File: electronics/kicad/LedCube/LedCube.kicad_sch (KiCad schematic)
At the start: 20 parts, among them J1 Conn_01x03, J2 Conn_01x03, J3 Conn_01x03, J4 Conn_01x04, J5 COM, J6 Conn_01x02, J7 JTAG, U1 ESP32-S3-DevKitC, U3 ESP32-DevKitM

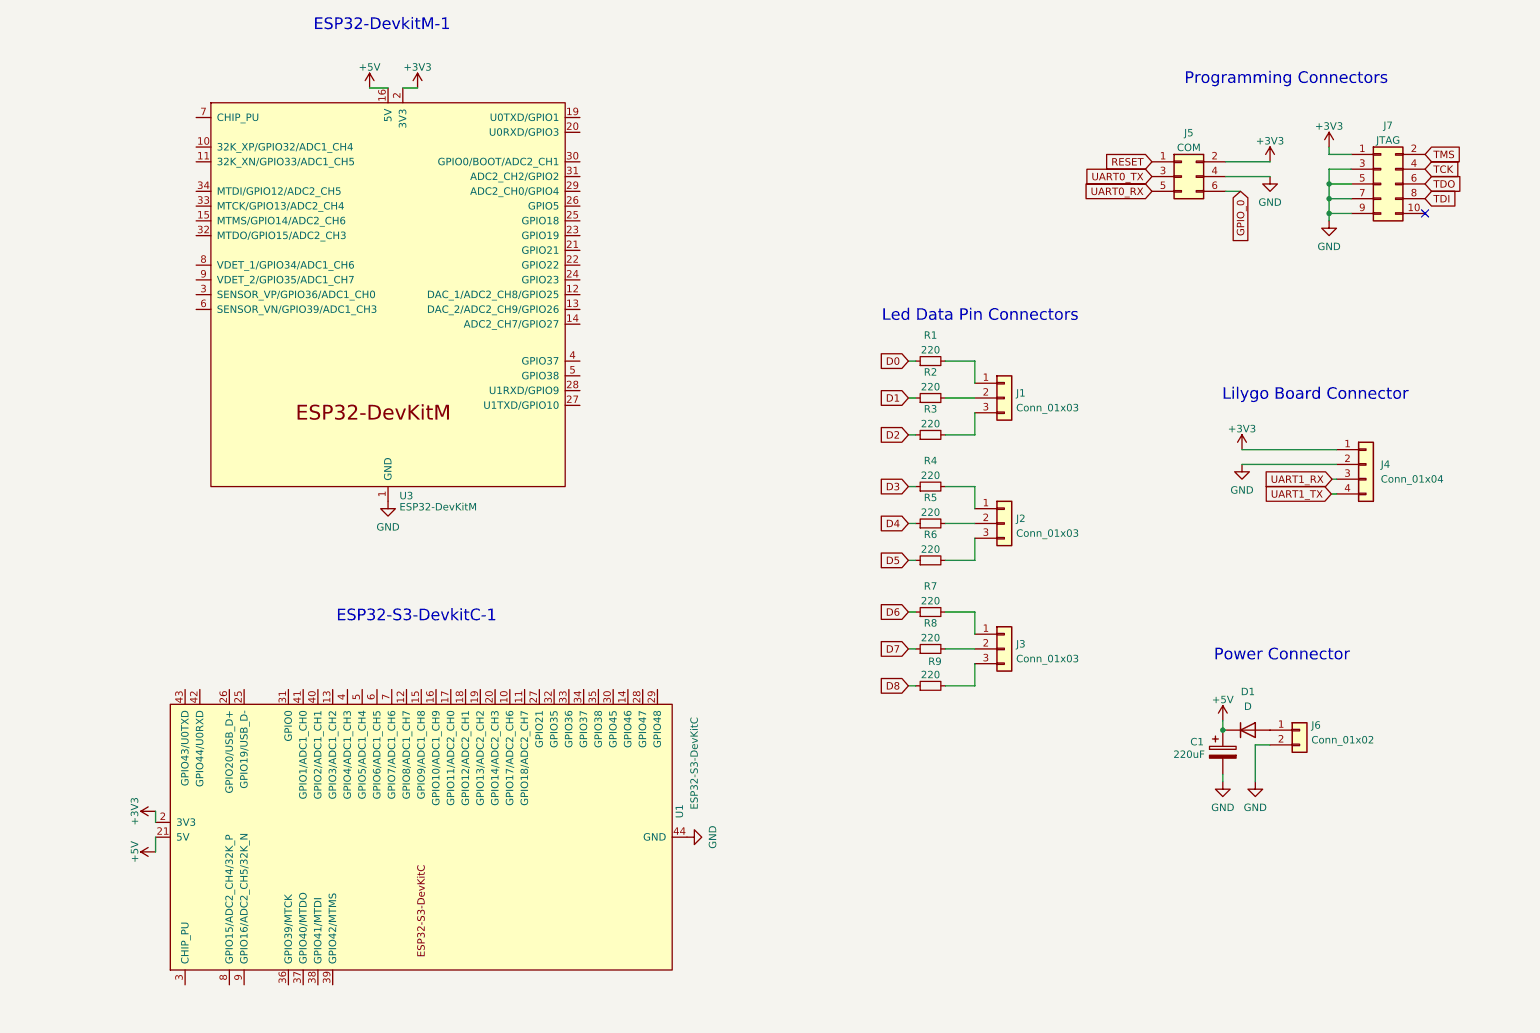
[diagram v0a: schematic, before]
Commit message: Finish KiCad PCB board
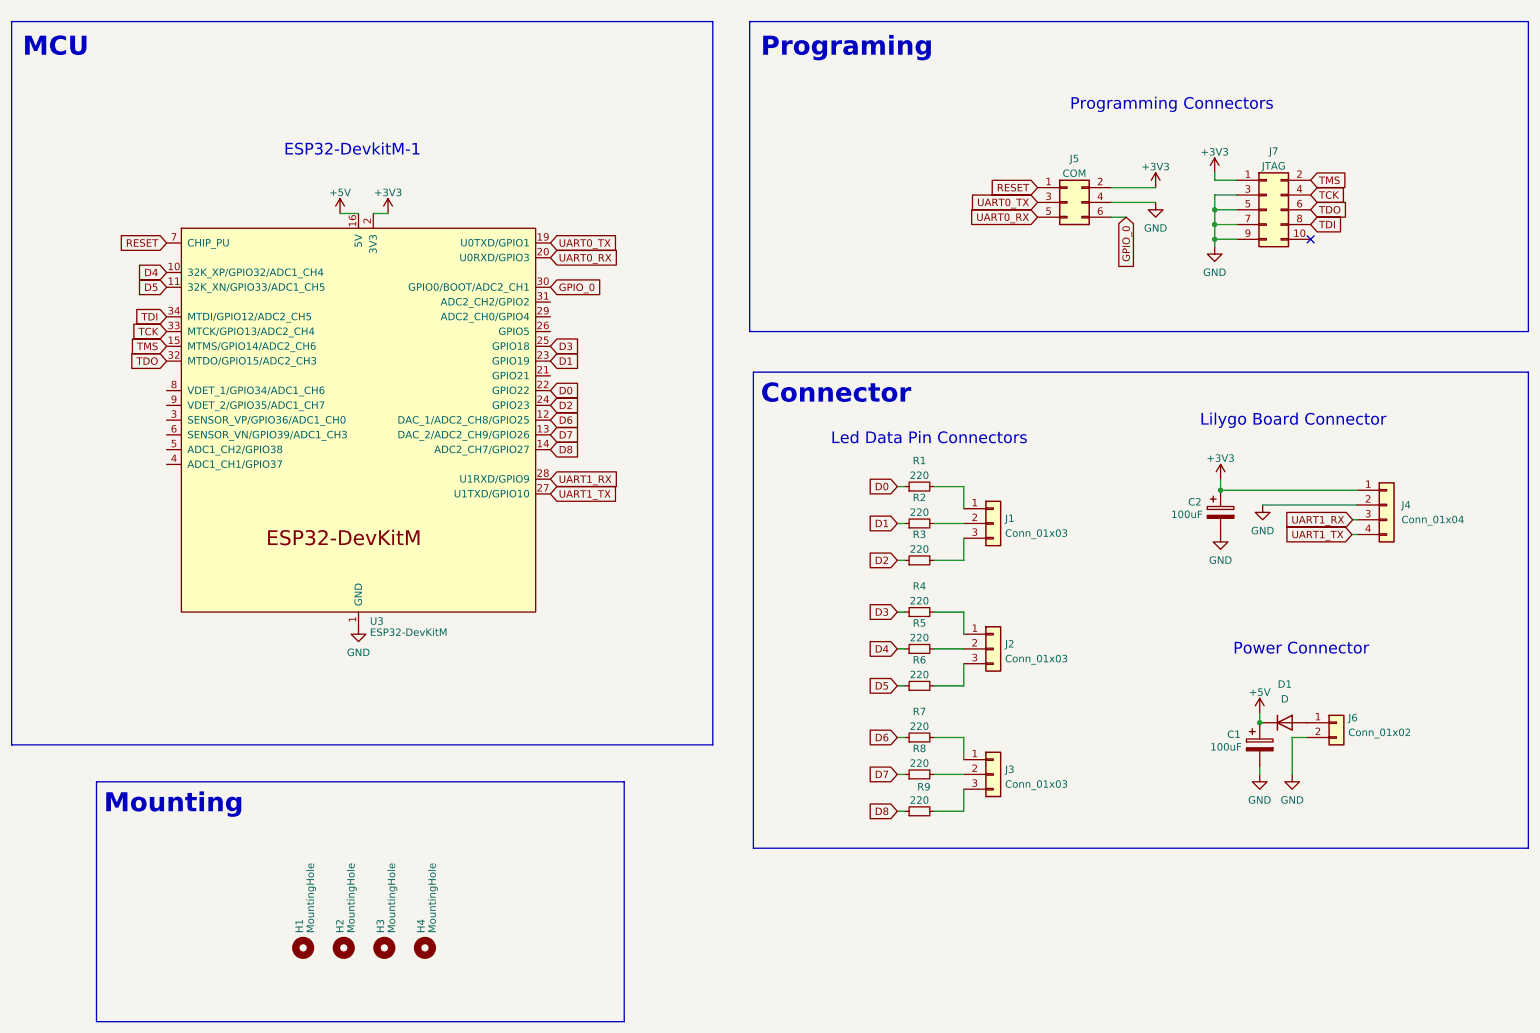
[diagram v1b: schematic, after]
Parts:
- removed U1: ESP32-S3-DevKitC, Espressif:ESP32-S3-DevKitC, symbol esp32:ESP32-S3-DevKitC
- added C2: 100uF, Capacitor_THT:C_Radial_D5.0mm_H5.0mm_P2.00mm, symbol Device:C_Polarized
- added H1, H2, H3, H4: MountingHole, MountingHole:MountingHole_3.2mm_M3_Pad, symbol Mechanical:MountingHole
- C1: value 220uF -> 100uF; footprint Capacitor_THT:C_Radial_D6.3mm_H5.0mm_P2.50mm -> Capacitor_THT:C_Radial_D5.0mm_H5.0mm_P2.00mm
- J5: footprint Connector_PinHeader_1.27mm:PinHeader_2x03_P1.27mm_Vertical -> Connectors:ESP_PROG_COM
- J6: footprint Connector_JST:JST_XH_B2B-XH-AM_1x02_P2.50mm_Vertical -> Connector_JST:JST_XH_B2B-XH-A_1x02_P2.50mm_Vertical
- J7: footprint Connector_PinHeader_1.27mm:PinHeader_2x05_P1.27mm_Vertical -> Connectors:ESP_PROG_JTAG
- U3: footprint Espressif:ESP32-DevKitC -> Espressif:ESP32-DevKitM
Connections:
- net +3V3: now also C2.1
- net D0: now also U3.22 (GPIO22)
- net D1: now also U3.23 (GPIO19)
- net D2: now also U3.24 (GPIO23)
- net D3: now also U3.25 (GPIO18)
- net D4: now also U3.10 (32K_XP/GPIO32/ADC1_CH4)
- net D5: now also U3.11 (32K_XN/GPIO33/ADC1_CH5)
- net D6: now also U3.12 (DAC_1/ADC2_CH8/GPIO25)
- net D7: now also U3.13 (DAC_2/ADC2_CH9/GPIO26)
- net D8: now also U3.14 (ADC2_CH7/GPIO27)
- net GND: now also C2.2
- net GPIO_0: now also U3.30 (GPIO0/BOOT/ADC2_CH1)
- net RESET: now also U3.7 (CHIP_PU)
- net TCK: now also U3.33 (MTCK/GPIO13/ADC2_CH4)
- net TDI: now also U3.34 (MTDI/GPIO12/ADC2_CH5)
- net TDO: now also U3.32 (MTDO/GPIO15/ADC2_CH3)
- net TMS: now also U3.15 (MTMS/GPIO14/ADC2_CH6)
- net UART0_RX: now also U3.20 (U0RXD/GPIO3)
- net UART0_TX: now also U3.19 (U0TXD/GPIO1)
- net UART1_RX: now also U3.28 (U1RXD/GPIO9)
- net UART1_TX: now also U3.27 (U1TXD/GPIO10)
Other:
- note added: "Connector"
- note added: "MCU"
- note added: "Mounting"
- note added: "Programing"
- note removed: "ESP32-S3-DevkitC-1"
- title: (none) -> Led Cube Board
- moved on the sheet: C1, D1, J1, J2, J3, J4, J5, J6, J7, R1, R2, R3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
